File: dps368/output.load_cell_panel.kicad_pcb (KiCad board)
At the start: 2 copper layers, 50 x 46 mm, 167 parts, among them J1 Conn_01x05_Female, U1 DPS368XTSA1

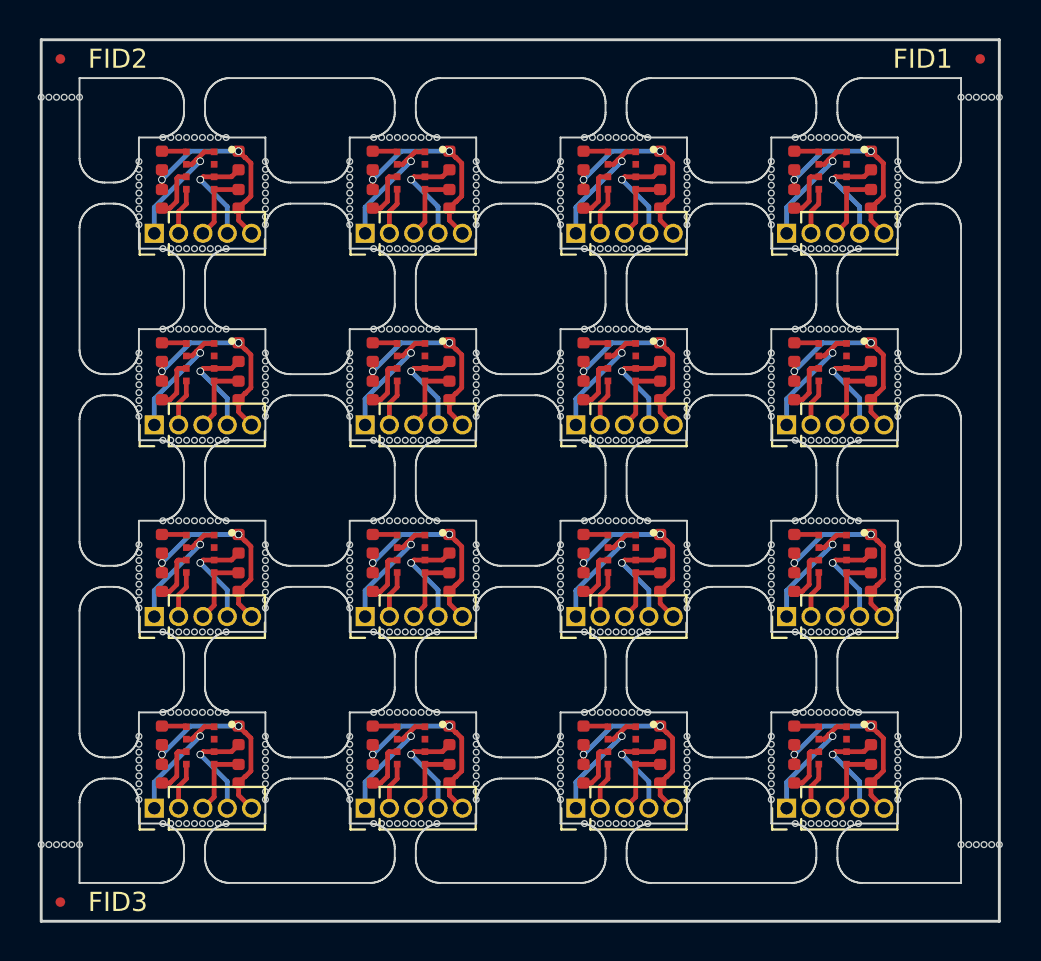
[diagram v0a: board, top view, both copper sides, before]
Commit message: goddamn it
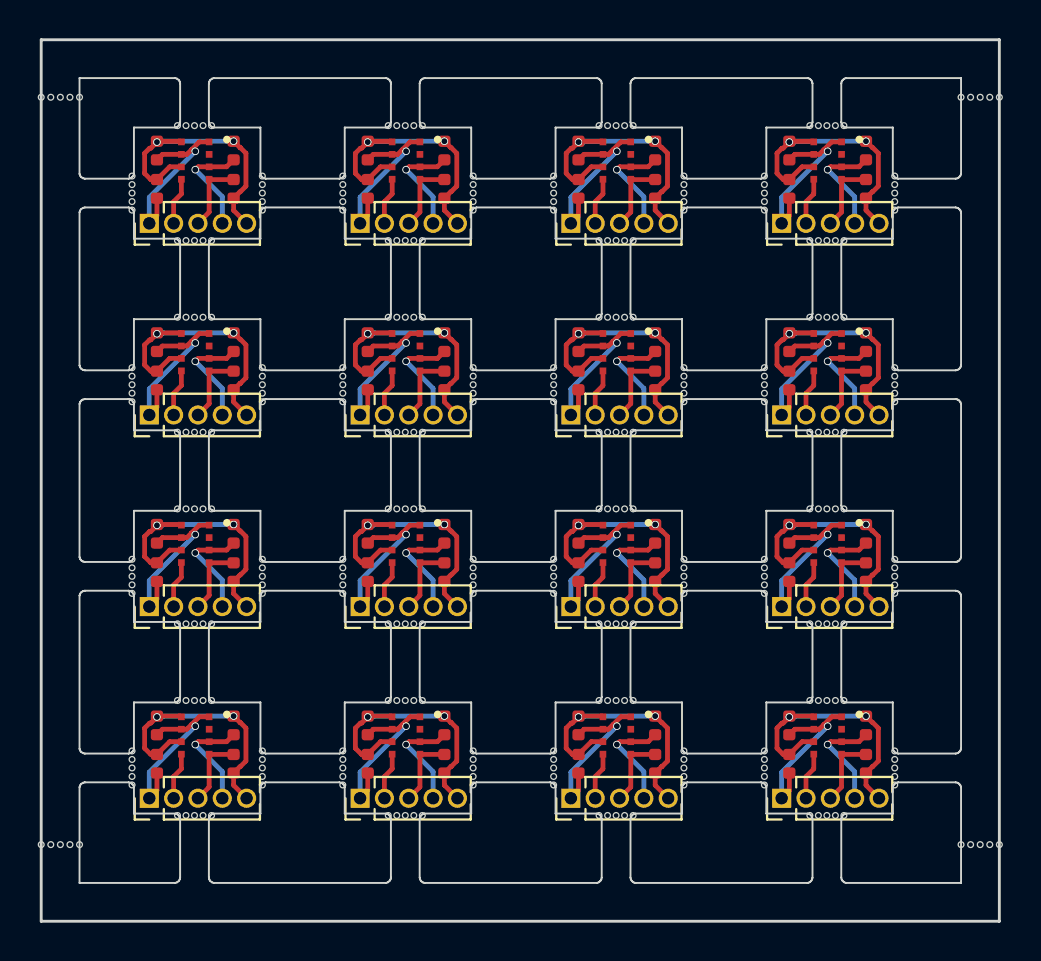
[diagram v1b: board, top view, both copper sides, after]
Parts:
- removed the ? at (141.1, 71.3)
- removed the ? at (156.6, 90.1)
- removed the ? at (134.6, 90.1)
- removed the ? at (131.3, 85.9)
- removed the ? at (131.3, 95.9)
- removed the ? at (134.6, 100.1)
- removed the ? at (142.3, 95.9)
- removed the ? at (145.6, 100.1)
- removed the ? at (142.3, 85.9)
- removed the ? at (145.6, 90.1)
- removed the ? at (141.1, 101.3)
- removed the ? at (136.7, 74.7)
- removed the ? at (136.7, 104.7)
- removed the ? at (152.1, 101.3)
- removed the ? at (147.7, 104.7)
- removed the ? at (158.7, 104.7)
- removed the ? at (163.1, 101.3)
- removed the ? at (164.3, 95.9)
- removed the ? at (167.6, 100.1)
- removed the ? at (164.3, 85.9)
- removed the ? at (167.6, 90.1)
- removed the ? at (164.3, 75.9)
- removed the ? at (152.1, 71.3)
- removed the ? at (167.6, 80.1)
- removed the ? at (153.3, 75.9)
- removed the ? at (156.6, 80.1)
- removed the ? at (145.6, 80.1)
- removed the ? at (142.3, 75.9)
- removed the ? at (131.3, 75.9)
- removed the ? at (134.6, 80.1)
- removed the ? at (130.1, 71.3)
- removed the ? at (158.7, 94.7)
- removed the ? at (163.1, 91.3)
- removed the ? at (147.7, 74.7)
- removed the ? at (147.7, 94.7)
- removed the ? at (152.1, 91.3)
- removed the ? at (136.7, 94.7)
- removed the ? at (141.1, 91.3)
- removed the ? at (141.1, 81.3)
- removed the ? at (136.7, 84.7)
- removed the ? at (152.1, 81.3)
- removed the ? at (147.7, 84.7)
- removed the ? at (163.1, 81.3)
- removed the ? at (158.7, 84.7)
- removed the ? at (163.1, 71.3)
- removed the ? at (169.7, 84.7)
- removed the ? at (169.7, 94.7)
- removed the ? at (169.7, 104.7)
- removed the ? at (164.3, 105.9)
- removed the ? at (153.3, 105.9)
- removed the ? at (142.3, 105.9)
- removed the ? at (131.3, 105.9)
- removed the ? at (130.1, 101.3)
- removed the ? at (130.1, 91.3)
- removed the ? at (130.1, 81.3)
- removed the ? at (158.7, 74.7)
- removed the ? at (134.6, 70.1)
- removed the ? at (145.6, 70.1)
- removed the ? at (156.6, 70.1)
- removed the ? at (167.6, 70.1)
- removed the ? at (169.7, 74.7)
- removed the ? at (153.3, 95.9)
- removed the ? at (156.6, 100.1)
- removed the ? at (153.3, 85.9)
- removed the C1 at (164.3, 101.3)
- removed the C1 at (153.3, 81.3)
- removed the C1 at (142.3, 81.3)
- removed the C1 at (131.3, 81.3)
- removed the C1 at (164.3, 71.3)
- removed the C1 at (153.3, 71.3)
- removed the C1 at (142.3, 71.3)
- removed the C1 at (153.3, 101.3)
- removed the C1 at (142.3, 101.3)
- removed the C1 at (131.3, 101.3)
- removed the C1 at (164.3, 91.3)
- removed the C1 at (153.3, 91.3)
- removed the C1 at (142.3, 91.3)
- removed the C1 at (131.3, 91.3)
- removed the C1 at (164.3, 81.3)
- removed the C2 at (164.3, 103.3)
- removed the C2 at (153.3, 83.3)
- removed the C2 at (142.3, 83.3)
- removed the C2 at (131.3, 83.3)
- removed the C2 at (164.3, 73.3)
- removed the C2 at (153.3, 73.3)
- removed the C2 at (142.3, 73.3)
- removed the C2 at (153.3, 103.3)
- removed the C2 at (142.3, 103.3)
- removed the C2 at (131.3, 103.3)
- removed the C2 at (164.3, 93.3)
- removed the C2 at (153.3, 93.3)
- removed the C2 at (142.3, 93.3)
- removed the C2 at (131.3, 93.3)
- removed the C2 at (164.3, 83.3)
- removed FID1, FID2, FID3: Fiducial_0.5mm_Dia_1mm_Outer, Fiducial:Fiducial_0.5mm_Dia_1mm_Outer
- removed the J1 at (163.9, 105.1)
- removed the J1 at (152.9, 85.1)
- removed the J1 at (141.9, 85.1)
- removed the J1 at (130.9, 85.1)
- removed the J1 at (163.9, 75.1)
- removed the J1 at (152.9, 75.1)
- removed the J1 at (141.9, 75.1)
- removed the J1 at (152.9, 105.1)
- removed the J1 at (141.9, 105.1)
- removed the J1 at (130.9, 105.1)
- removed the J1 at (163.9, 95.1)
- removed the J1 at (152.9, 95.1)
- removed the J1 at (141.9, 95.1)
- removed the J1 at (130.9, 95.1)
- removed the J1 at (163.9, 85.1)
- removed the R1 at (168.3, 103.3)
- removed the R1 at (157.3, 83.3)
- removed the R1 at (146.3, 83.3)
- removed the R1 at (135.3, 83.3)
- removed the R1 at (168.3, 73.3)
- removed the R1 at (157.3, 73.3)
- removed the R1 at (146.3, 73.3)
- removed the R1 at (157.3, 103.3)
- removed the R1 at (146.3, 103.3)
- removed the R1 at (135.3, 103.3)
- removed the R1 at (168.3, 93.3)
- removed the R1 at (157.3, 93.3)
- removed the R1 at (146.3, 93.3)
- removed the R1 at (135.3, 93.3)
- removed the R1 at (168.3, 83.3)
- removed the R2 at (168.3, 101.3)
- removed the R2 at (157.3, 81.3)
- removed the R2 at (146.3, 81.3)
- removed the R2 at (135.3, 81.3)
- removed the R2 at (168.3, 71.3)
- removed the R2 at (157.3, 71.3)
- removed the R2 at (146.3, 71.3)
- removed the R2 at (157.3, 101.3)
- removed the R2 at (146.3, 101.3)
- removed the R2 at (135.3, 101.3)
- removed the R2 at (168.3, 91.3)
- removed the R2 at (157.3, 91.3)
- removed the R2 at (146.3, 91.3)
- removed the R2 at (135.3, 91.3)
- removed the R2 at (168.3, 81.3)
- removed the U1 at (166.3, 101.8)
- removed the U1 at (155.3, 81.8)
- removed the U1 at (144.3, 81.8)
- removed the U1 at (133.3, 81.8)
- removed the U1 at (166.3, 71.8)
- removed the U1 at (155.3, 71.8)
- removed the U1 at (144.3, 71.8)
- removed the U1 at (155.3, 101.8)
- removed the U1 at (144.3, 101.8)
- removed the U1 at (133.3, 101.8)
- removed the U1 at (166.3, 91.8)
- removed the U1 at (155.3, 91.8)
- removed the U1 at (144.3, 91.8)
- removed the U1 at (133.3, 91.8)
- removed the U1 at (166.3, 81.8)
- added ?: , holes, F.Cu at (140.7, 72.1)
- added ?: , holes, F.Cu at (155.9, 89.5)
- added ?: , holes, F.Cu at (133.9, 89.5)
- added ?: , holes, F.Cu at (132.1, 85.5)
- added ?: , holes, F.Cu at (132.1, 95.5)
- added ?: , holes, F.Cu at (133.9, 99.5)
- added ?: , holes, F.Cu at (143.1, 95.5)
- added ?: , holes, F.Cu at (144.9, 99.5)
- added ?: , holes, F.Cu at (143.1, 85.5)
- added ?: , holes, F.Cu at (144.9, 89.5)
- added ?: , holes, F.Cu at (140.7, 102.1)
- added ?: , holes, F.Cu at (136.5, 73.9)
- added ?: , holes, F.Cu at (136.5, 103.9)
- added ?: , holes, F.Cu at (151.7, 102.1)
- added ?: , holes, F.Cu at (147.5, 103.9)
- added ?: , holes, F.Cu at (158.5, 103.9)
- added ?: , holes, F.Cu at (162.7, 102.1)
- added ?: , holes, F.Cu at (165.1, 95.5)
- added ?: , holes, F.Cu at (166.9, 99.5)
- added ?: , holes, F.Cu at (165.1, 85.5)
- added ?: , holes, F.Cu at (166.9, 89.5)
- added ?: , holes, F.Cu at (165.1, 75.5)
- added ?: , holes, F.Cu at (151.7, 72.1)
- added ?: , holes, F.Cu at (166.9, 79.5)
- added ?: , holes, F.Cu at (154.1, 75.5)
- added ?: , holes, F.Cu at (155.9, 79.5)
- added ?: , holes, F.Cu at (144.9, 79.5)
- added ?: , holes, F.Cu at (143.1, 75.5)
- added ?: , holes, F.Cu at (132.1, 75.5)
- added ?: , holes, F.Cu at (133.9, 79.5)
- added ?: , holes, F.Cu at (129.7, 72.1)
- added ?: , holes, F.Cu at (158.5, 93.9)
- added ?: , holes, F.Cu at (162.7, 92.1)
- added ?: , holes, F.Cu at (147.5, 73.9)
- added ?: , holes, F.Cu at (147.5, 93.9)
- added ?: , holes, F.Cu at (151.7, 92.1)
- added ?: , holes, F.Cu at (136.5, 93.9)
- added ?: , holes, F.Cu at (140.7, 92.1)
- added ?: , holes, F.Cu at (140.7, 82.1)
- added ?: , holes, F.Cu at (136.5, 83.9)
- added ?: , holes, F.Cu at (151.7, 82.1)
- added ?: , holes, F.Cu at (147.5, 83.9)
- added ?: , holes, F.Cu at (162.7, 82.1)
- added ?: , holes, F.Cu at (158.5, 83.9)
- added ?: , holes, F.Cu at (162.7, 72.1)
- added ?: , holes, F.Cu at (169.5, 83.9)
- added ?: , holes, F.Cu at (169.5, 93.9)
- added ?: , holes, F.Cu at (169.5, 103.9)
- added ?: , holes, F.Cu at (165.1, 105.5)
- added ?: , holes, F.Cu at (154.1, 105.5)
- added ?: , holes, F.Cu at (143.1, 105.5)
- added ?: , holes, F.Cu at (132.1, 105.5)
- added ?: , holes, F.Cu at (129.7, 102.1)
- added ?: , holes, F.Cu at (129.7, 92.1)
- added ?: , holes, F.Cu at (129.7, 82.1)
- added ?: , holes, F.Cu at (158.5, 73.9)
- added ?: , holes, F.Cu at (133.9, 69.5)
- added ?: , holes, F.Cu at (144.9, 69.5)
- added ?: , holes, F.Cu at (155.9, 69.5)
- added ?: , holes, F.Cu at (166.9, 69.5)
- added ?: , holes, F.Cu at (169.5, 73.9)
- added ?: , holes, F.Cu at (154.1, 95.5)
- added ?: , holes, F.Cu at (155.9, 99.5)
- added ?: , holes, F.Cu at (154.1, 85.5)
- added C1: 100n, Capacitor_SMD:C_0402_1005Metric, F.Cu at (164.0, 100.8)
- added C1: 100n, Capacitor_SMD:C_0402_1005Metric, F.Cu at (153.0, 80.8)
- added C1: 100n, Capacitor_SMD:C_0402_1005Metric, F.Cu at (142.0, 80.8)
- added C1: 100n, Capacitor_SMD:C_0402_1005Metric, F.Cu at (131.0, 80.8)
- added C1: 100n, Capacitor_SMD:C_0402_1005Metric, F.Cu at (164.0, 70.8)
- added C1: 100n, Capacitor_SMD:C_0402_1005Metric, F.Cu at (153.0, 70.8)
- added C1: 100n, Capacitor_SMD:C_0402_1005Metric, F.Cu at (142.0, 70.8)
- added C1: 100n, Capacitor_SMD:C_0402_1005Metric, F.Cu at (153.0, 100.8)
- added C1: 100n, Capacitor_SMD:C_0402_1005Metric, F.Cu at (142.0, 100.8)
- added C1: 100n, Capacitor_SMD:C_0402_1005Metric, F.Cu at (131.0, 100.8)
- added C1: 100n, Capacitor_SMD:C_0402_1005Metric, F.Cu at (164.0, 90.8)
- added C1: 100n, Capacitor_SMD:C_0402_1005Metric, F.Cu at (153.0, 90.8)
- added C1: 100n, Capacitor_SMD:C_0402_1005Metric, F.Cu at (142.0, 90.8)
- added C1: 100n, Capacitor_SMD:C_0402_1005Metric, F.Cu at (131.0, 90.8)
- added C1: 100n, Capacitor_SMD:C_0402_1005Metric, F.Cu at (164.0, 80.8)
- added C2: 100n, Capacitor_SMD:C_0402_1005Metric, F.Cu at (164.0, 102.8)
- added C2: 100n, Capacitor_SMD:C_0402_1005Metric, F.Cu at (153.0, 82.8)
- added C2: 100n, Capacitor_SMD:C_0402_1005Metric, F.Cu at (142.0, 82.8)
- added C2: 100n, Capacitor_SMD:C_0402_1005Metric, F.Cu at (131.0, 82.8)
- added C2: 100n, Capacitor_SMD:C_0402_1005Metric, F.Cu at (164.0, 72.8)
- added C2: 100n, Capacitor_SMD:C_0402_1005Metric, F.Cu at (153.0, 72.8)
- added C2: 100n, Capacitor_SMD:C_0402_1005Metric, F.Cu at (142.0, 72.8)
- added C2: 100n, Capacitor_SMD:C_0402_1005Metric, F.Cu at (153.0, 102.8)
- added C2: 100n, Capacitor_SMD:C_0402_1005Metric, F.Cu at (142.0, 102.8)
- added C2: 100n, Capacitor_SMD:C_0402_1005Metric, F.Cu at (131.0, 102.8)
- added C2: 100n, Capacitor_SMD:C_0402_1005Metric, F.Cu at (164.0, 92.8)
- added C2: 100n, Capacitor_SMD:C_0402_1005Metric, F.Cu at (153.0, 92.8)
- added C2: 100n, Capacitor_SMD:C_0402_1005Metric, F.Cu at (142.0, 92.8)
- added C2: 100n, Capacitor_SMD:C_0402_1005Metric, F.Cu at (131.0, 92.8)
- added C2: 100n, Capacitor_SMD:C_0402_1005Metric, F.Cu at (164.0, 82.8)
- added J1: Conn_01x05_Female, Connector_PinHeader_1.27mm:PinHeader_1x05_P1.27mm_Vertical, F.Cu at (163.6, 104.6)
- added J1: Conn_01x05_Female, Connector_PinHeader_1.27mm:PinHeader_1x05_P1.27mm_Vertical, F.Cu at (152.6, 84.6)
- added J1: Conn_01x05_Female, Connector_PinHeader_1.27mm:PinHeader_1x05_P1.27mm_Vertical, F.Cu at (141.6, 84.6)
- added J1: Conn_01x05_Female, Connector_PinHeader_1.27mm:PinHeader_1x05_P1.27mm_Vertical, F.Cu at (130.6, 84.6)
- added J1: Conn_01x05_Female, Connector_PinHeader_1.27mm:PinHeader_1x05_P1.27mm_Vertical, F.Cu at (163.6, 74.6)
- added J1: Conn_01x05_Female, Connector_PinHeader_1.27mm:PinHeader_1x05_P1.27mm_Vertical, F.Cu at (152.6, 74.6)
- added J1: Conn_01x05_Female, Connector_PinHeader_1.27mm:PinHeader_1x05_P1.27mm_Vertical, F.Cu at (141.6, 74.6)
- added J1: Conn_01x05_Female, Connector_PinHeader_1.27mm:PinHeader_1x05_P1.27mm_Vertical, F.Cu at (152.6, 104.6)
- added J1: Conn_01x05_Female, Connector_PinHeader_1.27mm:PinHeader_1x05_P1.27mm_Vertical, F.Cu at (141.6, 104.6)
- added J1: Conn_01x05_Female, Connector_PinHeader_1.27mm:PinHeader_1x05_P1.27mm_Vertical, F.Cu at (130.6, 104.6)
- added J1: Conn_01x05_Female, Connector_PinHeader_1.27mm:PinHeader_1x05_P1.27mm_Vertical, F.Cu at (163.6, 94.6)
- added J1: Conn_01x05_Female, Connector_PinHeader_1.27mm:PinHeader_1x05_P1.27mm_Vertical, F.Cu at (152.6, 94.6)
- added J1: Conn_01x05_Female, Connector_PinHeader_1.27mm:PinHeader_1x05_P1.27mm_Vertical, F.Cu at (141.6, 94.6)
- added J1: Conn_01x05_Female, Connector_PinHeader_1.27mm:PinHeader_1x05_P1.27mm_Vertical, F.Cu at (130.6, 94.6)
- added J1: Conn_01x05_Female, Connector_PinHeader_1.27mm:PinHeader_1x05_P1.27mm_Vertical, F.Cu at (163.6, 84.6)
- added R1: 10k, Resistor_SMD:R_0402_1005Metric, F.Cu at (168.0, 102.8)
- added R1: 10k, Resistor_SMD:R_0402_1005Metric, F.Cu at (157.0, 82.8)
- added R1: 10k, Resistor_SMD:R_0402_1005Metric, F.Cu at (146.0, 82.8)
- added R1: 10k, Resistor_SMD:R_0402_1005Metric, F.Cu at (135.0, 82.8)
- added R1: 10k, Resistor_SMD:R_0402_1005Metric, F.Cu at (168.0, 72.8)
- added R1: 10k, Resistor_SMD:R_0402_1005Metric, F.Cu at (157.0, 72.8)
- added R1: 10k, Resistor_SMD:R_0402_1005Metric, F.Cu at (146.0, 72.8)
- added R1: 10k, Resistor_SMD:R_0402_1005Metric, F.Cu at (157.0, 102.8)
- added R1: 10k, Resistor_SMD:R_0402_1005Metric, F.Cu at (146.0, 102.8)
- added R1: 10k, Resistor_SMD:R_0402_1005Metric, F.Cu at (135.0, 102.8)
- added R1: 10k, Resistor_SMD:R_0402_1005Metric, F.Cu at (168.0, 92.8)
- added R1: 10k, Resistor_SMD:R_0402_1005Metric, F.Cu at (157.0, 92.8)
- added R1: 10k, Resistor_SMD:R_0402_1005Metric, F.Cu at (146.0, 92.8)
- added R1: 10k, Resistor_SMD:R_0402_1005Metric, F.Cu at (135.0, 92.8)
- added R1: 10k, Resistor_SMD:R_0402_1005Metric, F.Cu at (168.0, 82.8)
- added R2: 10k, Resistor_SMD:R_0402_1005Metric, F.Cu at (168.0, 100.8)
- added R2: 10k, Resistor_SMD:R_0402_1005Metric, F.Cu at (157.0, 80.8)
- added R2: 10k, Resistor_SMD:R_0402_1005Metric, F.Cu at (146.0, 80.8)
- added R2: 10k, Resistor_SMD:R_0402_1005Metric, F.Cu at (135.0, 80.8)
- added R2: 10k, Resistor_SMD:R_0402_1005Metric, F.Cu at (168.0, 70.8)
- added R2: 10k, Resistor_SMD:R_0402_1005Metric, F.Cu at (157.0, 70.8)
- added R2: 10k, Resistor_SMD:R_0402_1005Metric, F.Cu at (146.0, 70.8)
- added R2: 10k, Resistor_SMD:R_0402_1005Metric, F.Cu at (157.0, 100.8)
- added R2: 10k, Resistor_SMD:R_0402_1005Metric, F.Cu at (146.0, 100.8)
- added R2: 10k, Resistor_SMD:R_0402_1005Metric, F.Cu at (135.0, 100.8)
- added R2: 10k, Resistor_SMD:R_0402_1005Metric, F.Cu at (168.0, 90.8)
- added R2: 10k, Resistor_SMD:R_0402_1005Metric, F.Cu at (157.0, 90.8)
- added R2: 10k, Resistor_SMD:R_0402_1005Metric, F.Cu at (146.0, 90.8)
- added R2: 10k, Resistor_SMD:R_0402_1005Metric, F.Cu at (135.0, 90.8)
- added R2: 10k, Resistor_SMD:R_0402_1005Metric, F.Cu at (168.0, 80.8)
- added U1: DPS368XTSA1, custom_lib:XDCR_DPS368XTSA1, F.Cu at (166.0, 101.3)
- added U1: DPS368XTSA1, custom_lib:XDCR_DPS368XTSA1, F.Cu at (155.0, 81.3)
- added U1: DPS368XTSA1, custom_lib:XDCR_DPS368XTSA1, F.Cu at (144.0, 81.3)
- added U1: DPS368XTSA1, custom_lib:XDCR_DPS368XTSA1, F.Cu at (133.0, 81.3)
- added U1: DPS368XTSA1, custom_lib:XDCR_DPS368XTSA1, F.Cu at (166.0, 71.3)
- added U1: DPS368XTSA1, custom_lib:XDCR_DPS368XTSA1, F.Cu at (155.0, 71.3)
- added U1: DPS368XTSA1, custom_lib:XDCR_DPS368XTSA1, F.Cu at (144.0, 71.3)
- added U1: DPS368XTSA1, custom_lib:XDCR_DPS368XTSA1, F.Cu at (155.0, 101.3)
- added U1: DPS368XTSA1, custom_lib:XDCR_DPS368XTSA1, F.Cu at (144.0, 101.3)
- added U1: DPS368XTSA1, custom_lib:XDCR_DPS368XTSA1, F.Cu at (133.0, 101.3)
- added U1: DPS368XTSA1, custom_lib:XDCR_DPS368XTSA1, F.Cu at (166.0, 91.3)
- added U1: DPS368XTSA1, custom_lib:XDCR_DPS368XTSA1, F.Cu at (155.0, 91.3)
- added U1: DPS368XTSA1, custom_lib:XDCR_DPS368XTSA1, F.Cu at (144.0, 91.3)
- added U1: DPS368XTSA1, custom_lib:XDCR_DPS368XTSA1, F.Cu at (133.0, 91.3)
- added U1: DPS368XTSA1, custom_lib:XDCR_DPS368XTSA1, F.Cu at (166.0, 81.3)
- moved C1 0.58 mm to (131.0, 70.8)
- moved C2 0.58 mm to (131.0, 72.8)
- moved J1 0.58 mm to (130.6, 74.6)
- moved R1 0.58 mm to (135.0, 72.8)
- moved R2 0.58 mm to (135.0, 70.8)
- moved U1 0.58 mm to (133.0, 71.3)
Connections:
- C1 pad 1: +3V3 -> GND
- C1 pad 2: Net-(C1-Pad2) -> +3V3
- C2 pad 1: Net-(C2-Pad1) -> GND
- U1 pad 6: Net-(C2-Pad1) -> +3V3
- U1 pad 8: Net-(C1-Pad2) -> +3V3
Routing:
- net +3V3: track 172.3 -> 235.8 mm
- net GND: track 107.3 -> 153.3 mm
- net Net-(C2-Pad1): track 42.5 -> 0.00 mm
- net Net-(C1-Pad2): track 20.6 -> 0.00 mm
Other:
- outline, holes or cut-outs redrawn
